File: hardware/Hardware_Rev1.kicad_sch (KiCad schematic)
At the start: 134 parts, among them J1 RJ45_LED_Shielded, J2 6P6C, U3 OKI, U5 TSR_1-2450, U6 Teensy4.1_DEV-16771

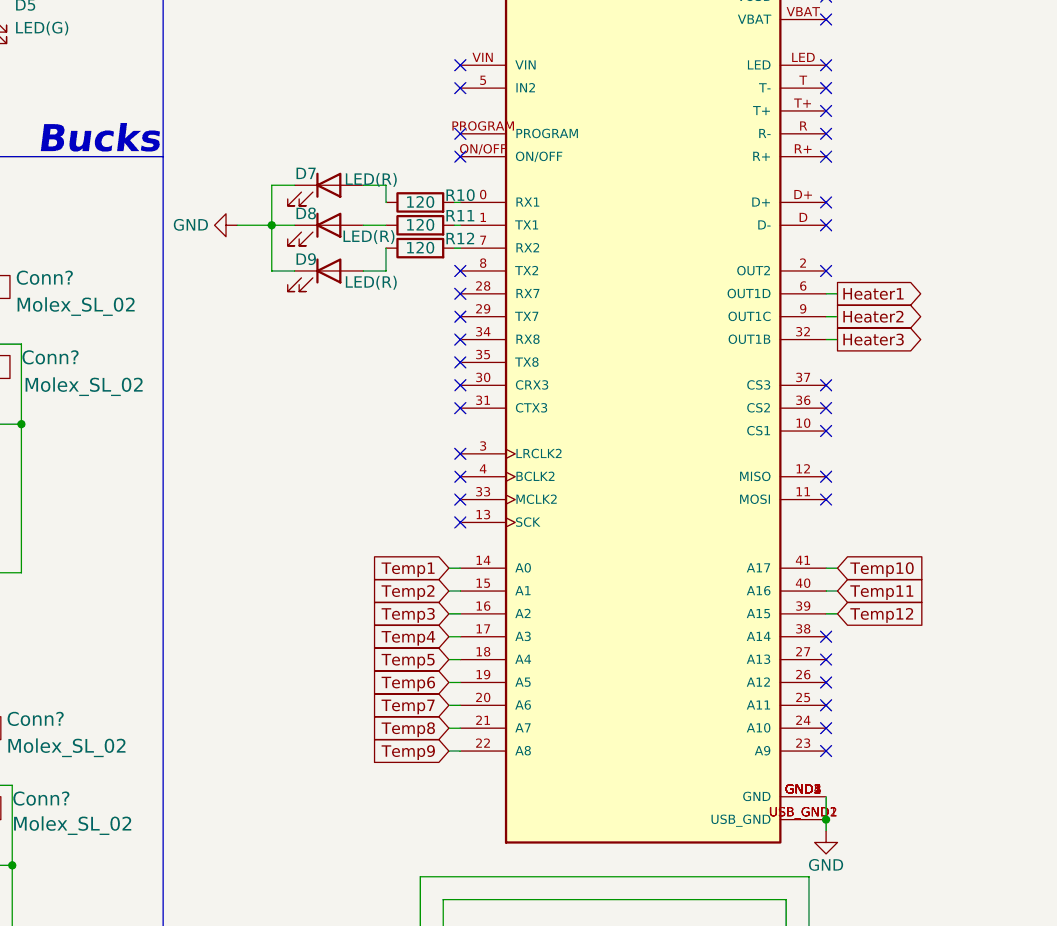
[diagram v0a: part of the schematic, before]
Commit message: done with schematic ?
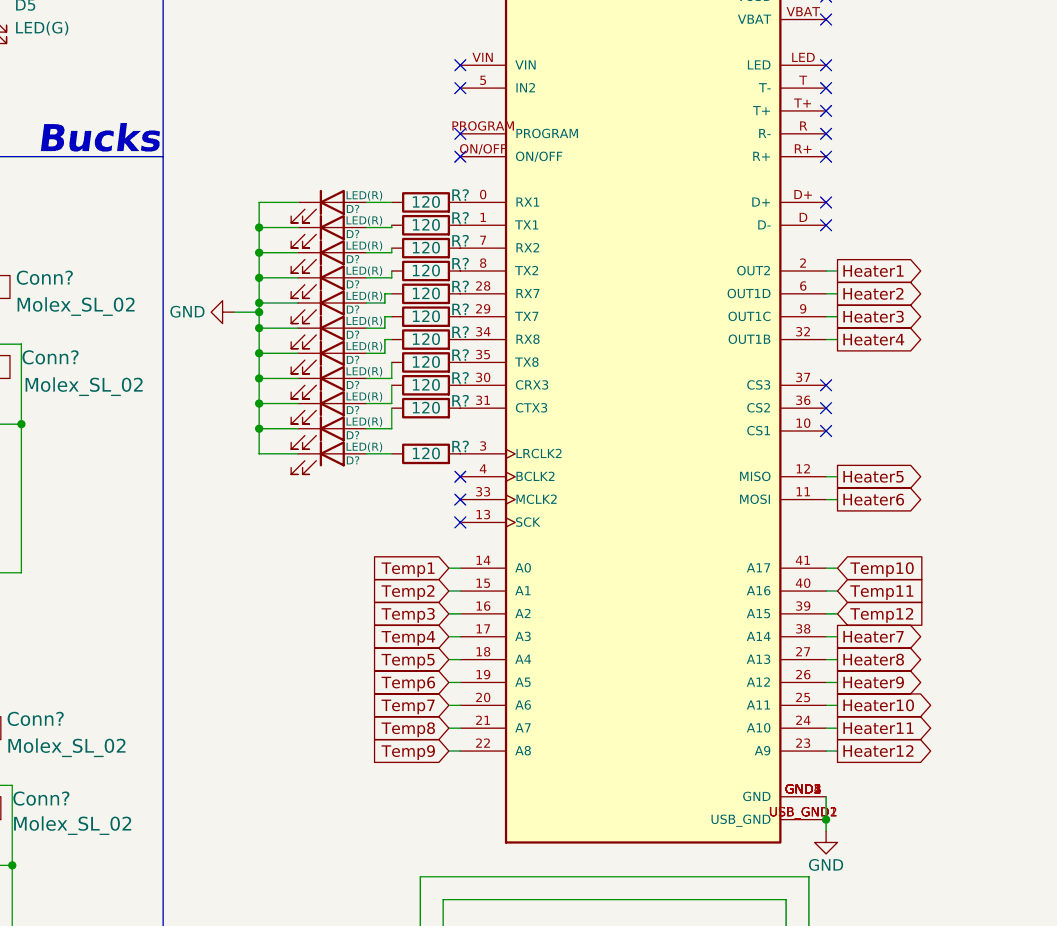
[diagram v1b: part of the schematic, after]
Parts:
- removed D7, D8, D9: LED(R), LED_SMD:LED_0603_1608Metric_Pad1.05x0.95mm_HandSolder, symbol Device:LED
- removed R10, R11, R12: 120, Resistor_SMD:R_0603_1608Metric_Pad0.98x0.95mm_HandSolder, symbol Device:R
- added D? (x11): LED(R), LED_SMD:LED_0603_1608Metric_Pad1.05x0.95mm_HandSolder, symbol Device:LED
- added R? (x11): 120, symbol Device:R
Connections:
- net GND: now also D?.1 (K), D?.1 (K), D?.1 (K), D?.1 (K), D?.1 (K), D?.1 (K), D?.1 (K), D?.1 (K), D?.1 (K), D?.1 (K), D?.1 (K)
- net Heater1: now also U6.2 (OUT2); no longer U6.6 (OUT1D)
- net Heater10: now also U6.25 (A11)
- net Heater11: now also U6.24 (A10)
- net Heater12: now also U6.23 (A9)
- net Heater2: now also U6.6 (OUT1D); no longer U6.9 (OUT1C)
- net Heater3: now also U6.9 (OUT1C); no longer U6.32 (OUT1B)
- net Heater4: now also U6.32 (OUT1B)
- net Heater5: now also U6.12 (MISO)
- net Heater6: now also U6.11 (MOSI)
- net Heater7: now also U6.38 (A14)
- net Heater8: now also U6.27 (A13)
- net Heater9: now also U6.26 (A12)
- net at U6.0 (RX1): now also R?.2
- net at U6.1 (TX1): now also R?.2
- net at U6.28 (RX7): now also R?.2
- net at U6.29 (TX7): now also R?.2
- net at U6.3 (LRCLK2): now also R?.2
- net at U6.30 (CRX3): now also R?.2
- net at U6.31 (CTX3): now also R?.2
- net at U6.34 (RX8): now also R?.2
- net at U6.35 (TX8): now also R?.2
- net at U6.7 (RX2): now also R?.2
- net at U6.8 (TX2): now also R?.2
- new net: D?.2 (A), R?.1 (x11)
- no-connect marks 40 -> 23
